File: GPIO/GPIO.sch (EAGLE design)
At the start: 30 parts

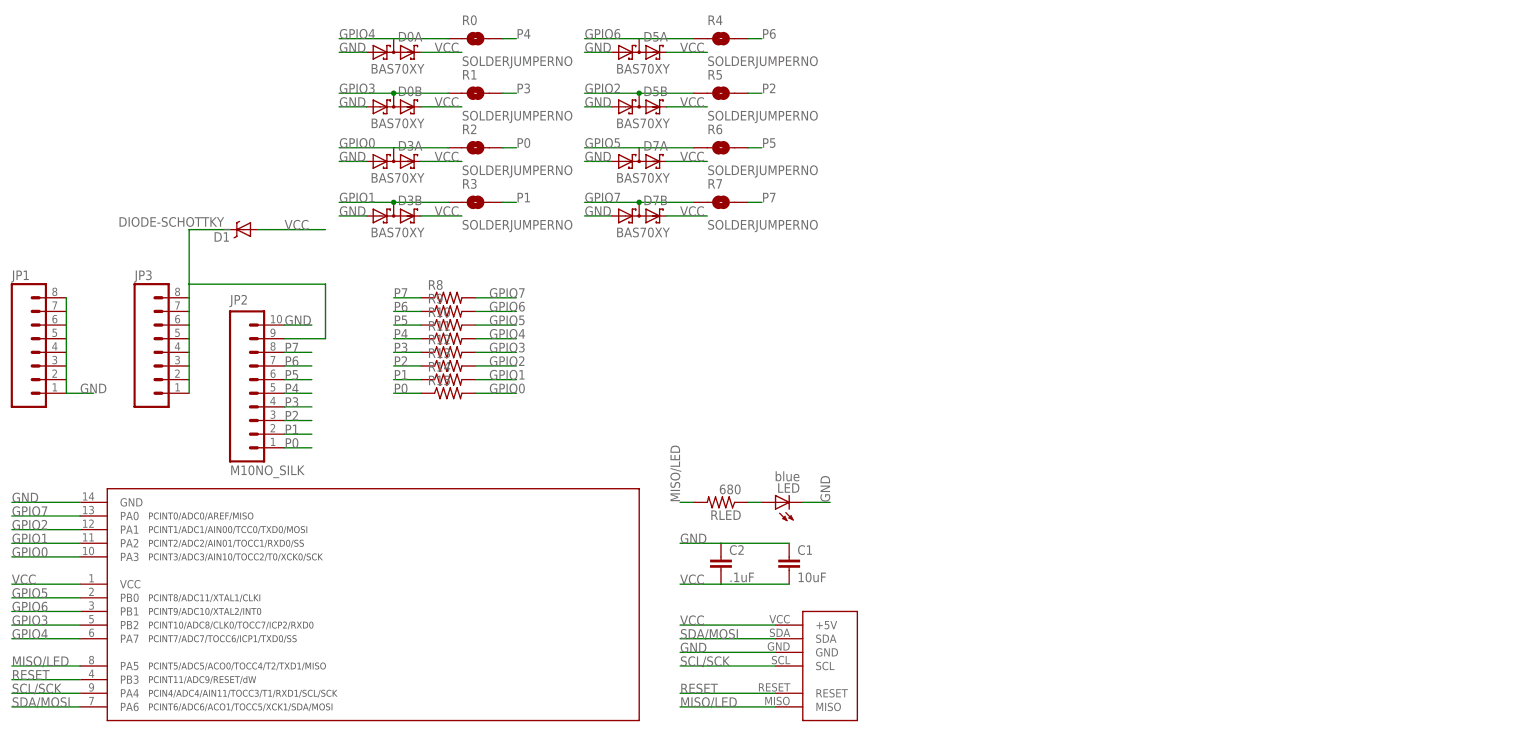
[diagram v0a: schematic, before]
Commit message: Latest version of schematics and boards
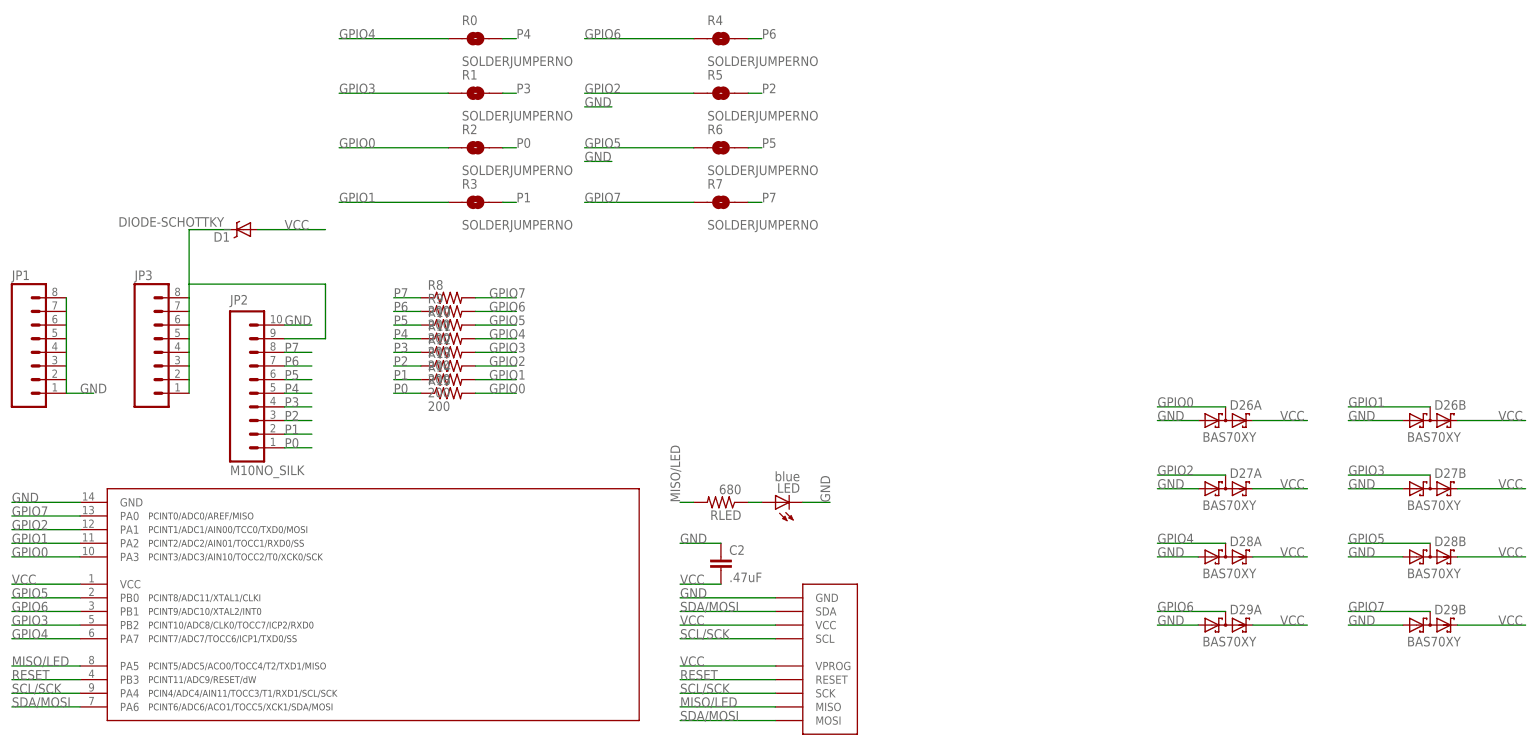
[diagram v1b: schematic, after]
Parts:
- removed C1: 10uF, SparkFun-Capacitors:CAP0805
- removed D0, D3, D5, D7: BAS70XY, diode:BAS70XY
- added D26, D27, D28, D29: BAS70XY, diode:BAS70XY
- C2: value .1uF -> .47uF
- R10, R11, R12, R13, R14, R15, R8, R9: value (none) -> 200; device adafruit:R-US_R0805 -> SparkFun-Resistors:RESISTOR0805-RES
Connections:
- net GND: now also D26A.A1, D26B.A1, D27A.A1, D27B.A1, D28A.A1, D28B.A1, D29A.A1, D29B.A1; no longer C1.1, D0A.A1, D0B.A1, D3A.A1, D3B.A1, D5A.A1, D5B.A1, D7A.A1, D7B.A1
- net GPIO0: now also D26A.C1A2; no longer D3A.C1A2
- net GPIO1: now also D26B.C1A2; no longer D3B.C1A2
- net GPIO2: now also D27A.C1A2; no longer D5B.C1A2
- net GPIO3: now also D27B.C1A2; no longer D0B.C1A2
- net GPIO4: now also D28A.C1A2; no longer D0A.C1A2
- net GPIO5: now also D28B.C1A2; no longer D7A.C1A2
- net GPIO6: now also D29A.C1A2; no longer D5A.C1A2
- net GPIO7: now also D29B.C1A2; no longer D7B.C1A2
- net SCL/SCK: now also U$4.SCK
- net SDA/MOSI: now also U$4.MOSI
- net VCC: now also D26A.C2, D26B.C2, D27A.C2, D27B.C2, D28A.C2, D28B.C2, D29A.C2, D29B.C2, U$4.VCC, U$4.VPROG; no longer C1.2, D0A.C2, D0B.C2, D3A.C2, D3B.C2, D5A.C2, D5B.C2, D7A.C2, D7B.C2, U$4.+5V
